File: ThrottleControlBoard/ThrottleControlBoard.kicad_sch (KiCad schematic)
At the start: 85 parts, among them J1 BTS7960 module, J10 Conn_01x04, J11 Conn_01x04, J12 Conn_01x02, J13 Conn_01x02, J2 e-Throttle, J3 Conn_01x14, J4 TB TPS, J5 5V, J6 AUX, J7 AUX, J8 AUX, J9 AUX, SW2 SW_SPDT, U1 PCA9685PW

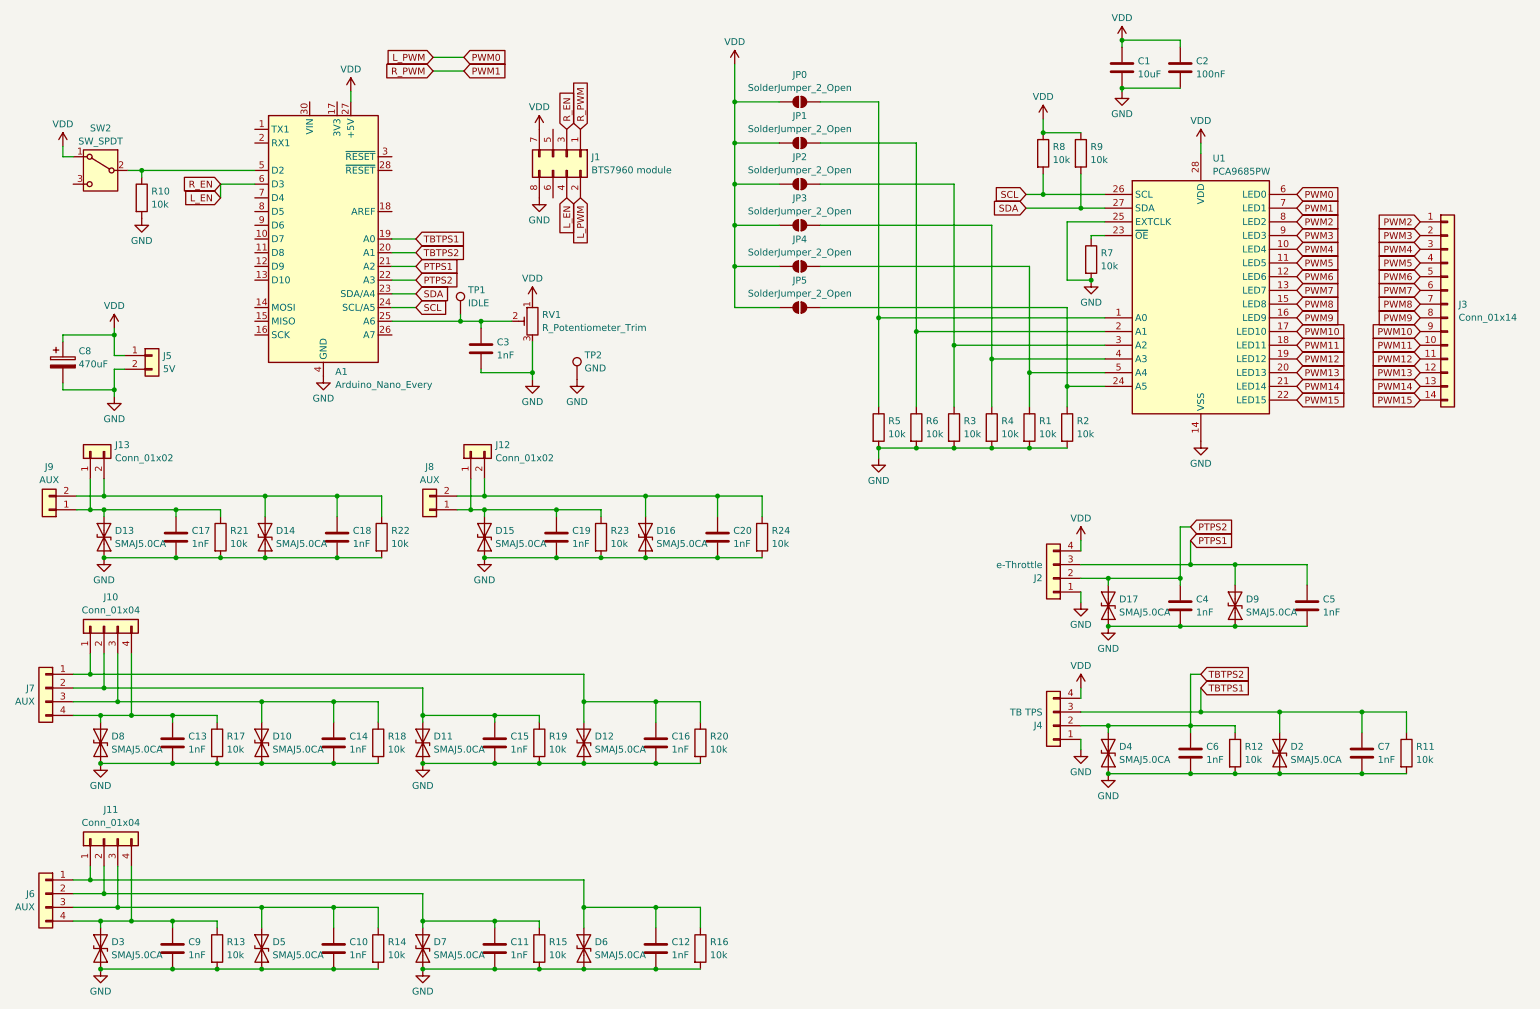
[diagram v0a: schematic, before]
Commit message: pcb done
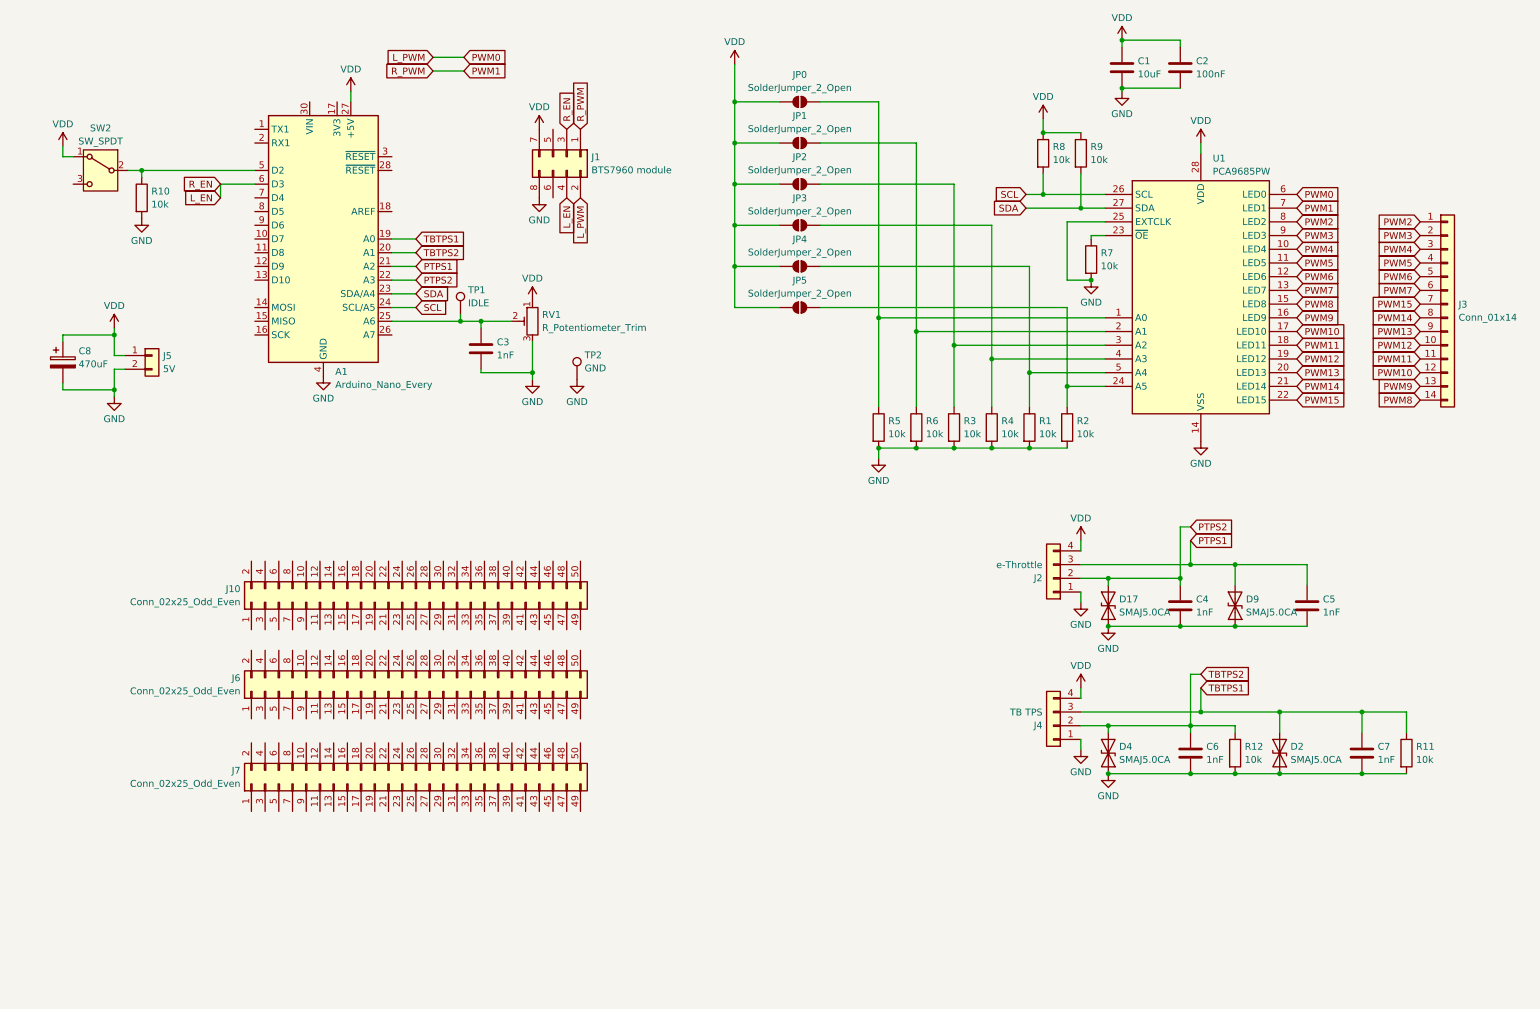
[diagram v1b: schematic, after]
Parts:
- removed C10, C11, C12, C13, C14, C15, C16, C17, C18, C19, C20, C9: 1nF, Capacitor_SMD:C_0805_2012Metric_Pad1.18x1.45mm_HandSolder, symbol Device:C
- removed D10, D11, D12, D13, D14, D15, D16, D3, D5, D6, D7, D8: SMAJ5.0CA, Diode_SMD:D_SMA, symbol Diode:SMAJ5.0CA
- removed J10, J11: Conn_01x04, Connector_PinHeader_2.54mm:PinHeader_1x04_P2.54mm_Vertical, symbol Connector_Generic:Conn_01x04
- removed J12, J13: Conn_01x02, Connector_PinHeader_2.54mm:PinHeader_1x02_P2.54mm_Vertical, symbol Connector_Generic:Conn_01x02
- removed J6, J7: AUX, TerminalBlock:TerminalBlock_Altech_AK300-4_P5.00mm, symbol Connector_Generic:Conn_01x04
- removed J8, J9: AUX, TerminalBlock:TerminalBlock_Altech_AK300-2_P5.00mm, symbol Connector_Generic:Conn_01x02
- removed R13, R14, R15, R16, R17, R18, R19, R20, R21, R22, R23, R24: 10k, Resistor_SMD:R_0603_1608Metric_Pad0.98x0.95mm_HandSolder, symbol Device:R
- added J10, J6, J7: Conn_02x25_Odd_Even, Connector_PinHeader_2.54mm:PinHeader_2x25_P2.54mm_Vertical, symbol Connector_Generic:Conn_02x25_Odd_Even
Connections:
- net PWM10: now also J3.12 (Pin_12); no longer J3.9 (Pin_9)
- net PWM11: now also J3.11 (Pin_11); no longer J3.10 (Pin_10)
- net PWM12: now also J3.10 (Pin_10); no longer J3.11 (Pin_11)
- net PWM13: now also J3.9 (Pin_9); no longer J3.12 (Pin_12)
- net PWM14: now also J3.8 (Pin_8); no longer J3.13 (Pin_13)
- net PWM15: now also J3.7 (Pin_7); no longer J3.14 (Pin_14)
- net PWM8: now also J3.14 (Pin_14); no longer J3.7 (Pin_7)
- net PWM9: now also J3.13 (Pin_13); no longer J3.8 (Pin_8)
